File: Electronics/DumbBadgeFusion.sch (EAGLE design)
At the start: 139 parts, among them IC1 74245MTC, IC2 74245MTC, IC3 74245MTC, SW1 SPST_TACT-KMR2, T1 MMUN2133LT1G, U1 TDP3E001DRLR-SOT-23-5SOT-23-5, U2 TPS61090RSAR, U3 MCP73871, U4 FAN5333BSX, U6 MAX3232, X4 32.768

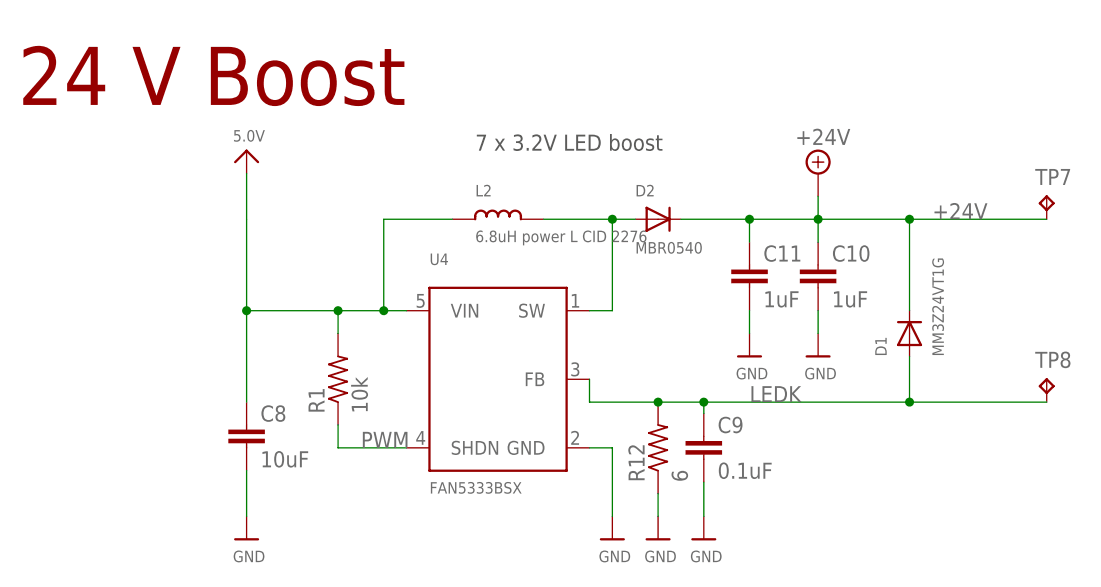
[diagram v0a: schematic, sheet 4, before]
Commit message: more power supply
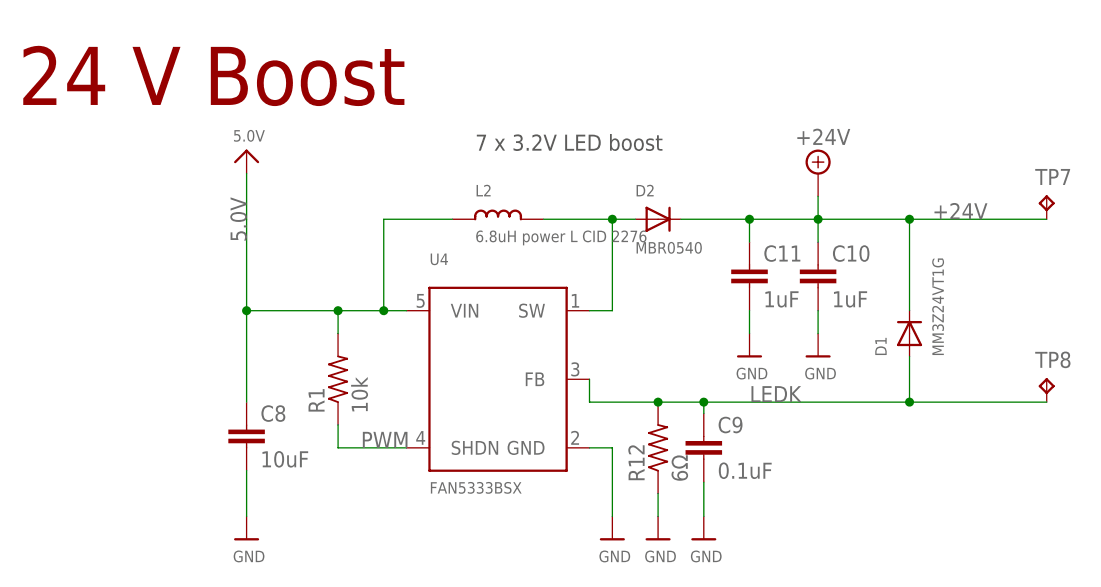
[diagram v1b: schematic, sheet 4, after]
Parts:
- R12: value 6 -> 6Ω
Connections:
- removed net N$21: C8.1, L2.1, R1.2, U4.VIN
- net 5.0V: now also C8.1, L2.1, R1.2, U4.VIN
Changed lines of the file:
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@@
 <part name="C11" library="SparkFun-Capacitors" library_urn="urn:adsk.eagle:library:510" deviceset="0.1UF" device="-0603-25V-(+80/-20%)" package3d_urn="urn:adsk.eagle:package:37414/1" value="1uF"/>
 <part name="R1" library="adafruit" deviceset="R-US_" device="R0603" value="10k"/>
-<part name="R12" library="adafruit" deviceset="R-US_" device="R0603" value="6"/>
+<part name="R12" library="adafruit" deviceset="R-US_" device="R0603" value="6Ω"/>
 <part name="U$33" library="microbuilder" deviceset="5.0V" device=""/>
 <part name="U$30" library="FPC" deviceset="50PINFPC" device=""/>
@@
 <wire x1="33.02" y1="152.4" x2="33.02" y2="157.48" width="0.1524" layer="91"/>
 </segment>
+<segment>
+<wire x1="33.02" y1="142.24" x2="33.02" y2="132.08" width="0.1524" layer="91"/>
+<wire x1="50.8" y1="142.24" x2="48.26" y2="142.24" width="0.1524" layer="91"/>
+<wire x1="48.26" y1="142.24" x2="43.18" y2="142.24" width="0.1524" layer="91"/>
+<wire x1="43.18" y1="142.24" x2="33.02" y2="142.24" width="0.1524" layer="91"/>
+<wire x1="48.26" y1="142.24" x2="48.26" y2="152.4" width="0.1524" layer="91"/>
+<wire x1="48.26" y1="152.4" x2="55.88" y2="152.4" width="0.1524" layer="91"/>
+<junction x="48.26" y="142.24"/>
+<pinref part="U4" gate="G$1" pin="VIN"/>
+<pinref part="L2" gate="G$1" pin="1"/>
+<pinref part="C8" gate="G$1" pin="1"/>
+<pinref part="R1" gate="G$1" pin="2"/>
+<wire x1="43.18" y1="139.7" x2="43.18" y2="142.24" width="0.1524" layer="91"/>
+<junction x="43.18" y="142.24"/>
+<wire x1="33.02" y1="142.24" x2="33.02" y2="152.4" width="0.1524" layer="91"/>
+<junction x="33.02" y="142.24"/>
+<label x="33.02" y="149.86" size="1.778" layer="95" rot="R90"/>
+</segment>
 </net>
 <net name="LEDK" class="0">
@@
 </segment>
 </net>
-<net name="N$21" class="0">
-<segment>
-<wire x1="33.02" y1="142.24" x2="33.02" y2="132.08" width="0.1524" layer="91"/>
-<wire x1="50.8" y1="142.24" x2="48.26" y2="142.24" width="0.1524" layer="91"/>
-<wire x1="48.26" y1="142.24" x2="43.18" y2="142.24" width="0.1524" layer="91"/>
-<wire x1="43.18" y1="142.24" x2="33.02" y2="142.24" width="0.1524" layer="91"/>
-<wire x1="48.26" y1="142.24" x2="48.26" y2="152.4" width="0.1524" layer="91"/>
-<wire x1="48.26" y1="152.4" x2="55.88" y2="152.4" width="0.1524" layer="91"/>
-<junction x="48.26" y="142.24"/>
-<pinref part="U4" gate="G$1" pin="VIN"/>
-<pinref part="L2" gate="G$1" pin="1"/>
-<pinref part="C8" gate="G$1" pin="1"/>
-<pinref part="R1" gate="G$1" pin="2"/>
-<wire x1="43.18" y1="139.7" x2="43.18" y2="142.24" width="0.1524" layer="91"/>
-<junction x="43.18" y="142.24"/>
-<wire x1="33.02" y1="142.24" x2="33.02" y2="152.4" width="0.1524" layer="91"/>
-<junction x="33.02" y="142.24"/>
-</segment>
-</net>
